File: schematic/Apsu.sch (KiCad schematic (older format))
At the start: 0 parts

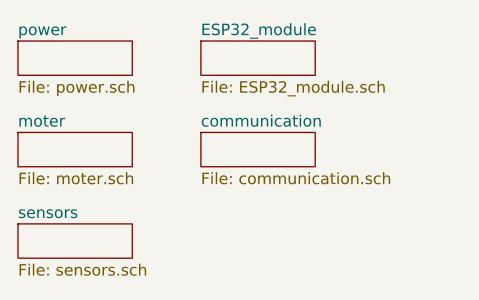
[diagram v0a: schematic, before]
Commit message: power on seperate board
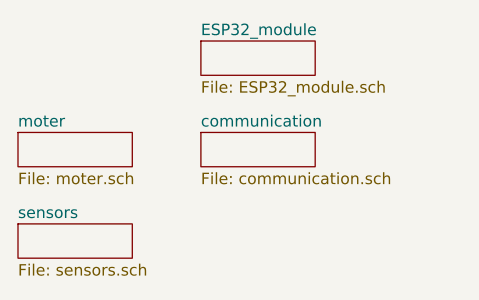
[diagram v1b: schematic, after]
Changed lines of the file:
@@
 $Descr A4 11693 8268
 encoding utf-8
-Sheet 1 6
+Sheet 1 5
 Title ""
 Date ""
@@
 $EndSheet
 $Sheet
-S 800  800  500  150
-U 5EEC6D97
-F0 "power" 50
-F1 "power.sch" 50
-$EndSheet
-$Sheet
